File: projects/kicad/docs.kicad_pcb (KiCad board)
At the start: 2 copper layers, 123.5 x 99.6 mm, 19 parts, among them SW1 SW_PUSH, SW2 SW_PUSH, SW3 SW_PUSH, SW4 SW_PUSH, SW5 SW_PUSH, SW6 SW_PUSH, SW7 RotaryEncoder_Switch, U2 LCD

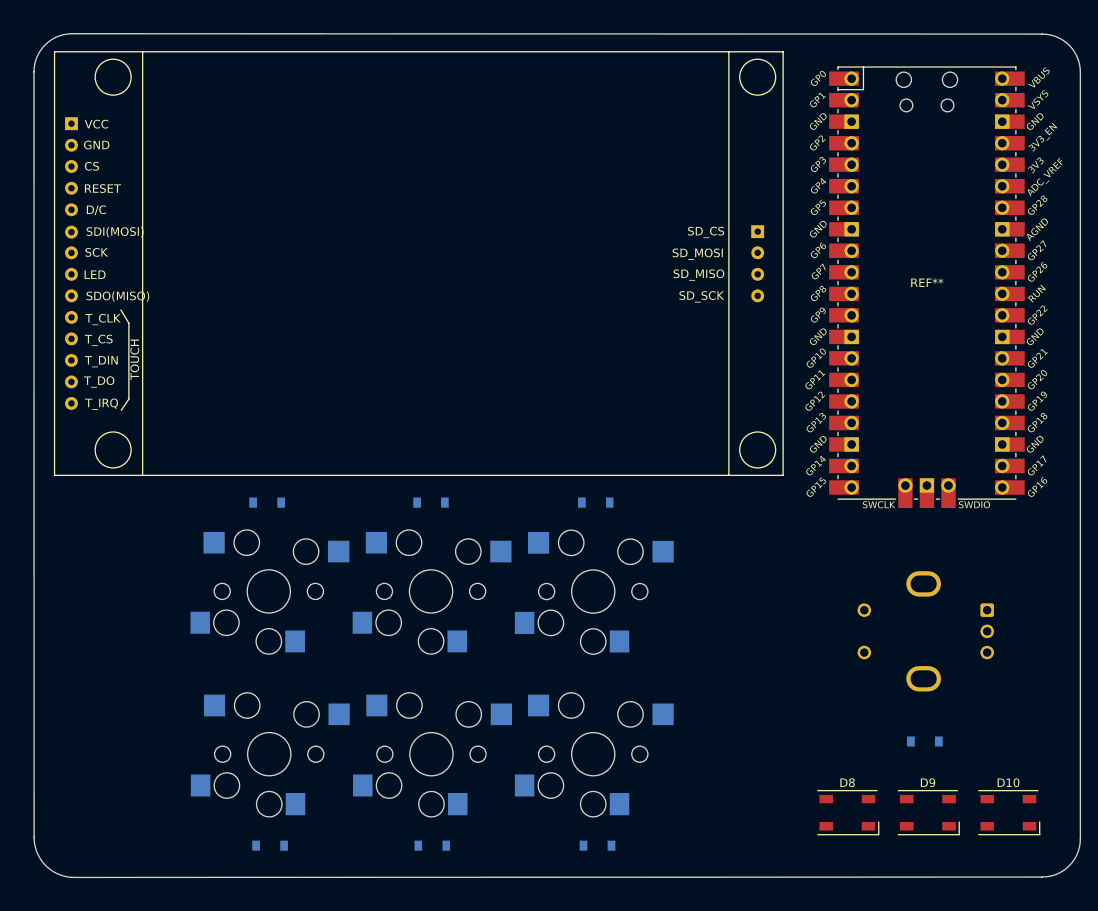
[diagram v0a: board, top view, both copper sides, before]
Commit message: Update_0128
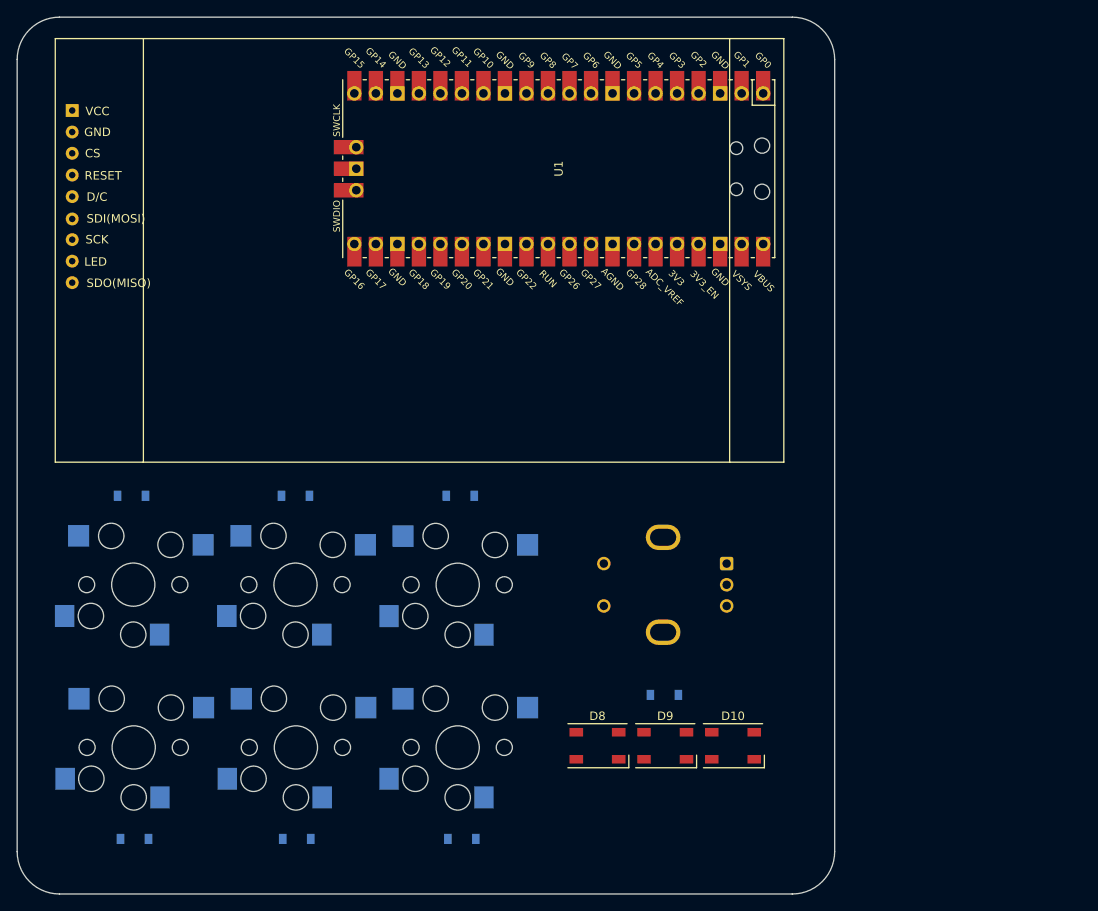
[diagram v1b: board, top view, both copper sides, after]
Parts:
- removed REF**: RPi_Pico_SMD_TH, KiCAD_RP_Pico:RPi_Pico_SMD_TH
- removed U2: LCD, tft_displays:2.8_tft_240x320_touch_sd_spi
- added U1: Pico, KiCad-RP-Pico-main:RPi_Pico_SMD_TH, F.Cu at (149.4, 39.4)
- added U3: 2.8_240x320_touch_sd_spi, original_tft_display:2.8_tft_240x320_touch_sd_spi, F.Cu at (176.0, 24.0)
- moved D10 33.4 mm to (170.0, 107.5)
- moved D9 32.0 mm to (162.0, 107.5)
- moved D7 31.2 mm to (161.9, 101.5)
- moved SW7 31.2 mm to (169.2, 86.0)
- moved D8 30.5 mm to (154.0, 107.5)
- moved D1 16.0 mm to (99.0, 78.0)
- moved D2 16.0 mm to (99.3, 118.5)
- moved D3 16.0 mm to (118.3, 78.0)
- moved D4 16.0 mm to (118.5, 118.5)
- moved D5 16.0 mm to (137.8, 78.0)
- moved D6 16.0 mm to (138.0, 118.5)
- moved SW1 16.0 mm to (99.2, 88.5)
- moved SW2 16.0 mm to (99.3, 107.7)
- moved SW3 16.0 mm to (118.4, 88.5)
- moved SW4 16.0 mm to (118.4, 107.7)
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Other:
- board size 123.5 x 99.6 mm -> 96.5 x 103.5 mm
